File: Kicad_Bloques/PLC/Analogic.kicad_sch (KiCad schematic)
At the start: 1 part, among them U5 LM324A

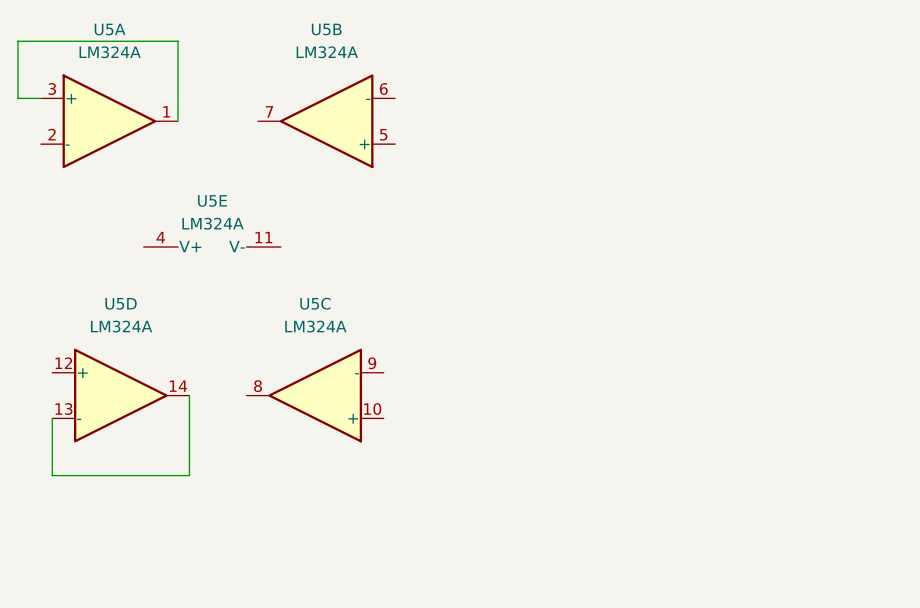
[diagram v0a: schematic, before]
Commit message: Bloque Analogico
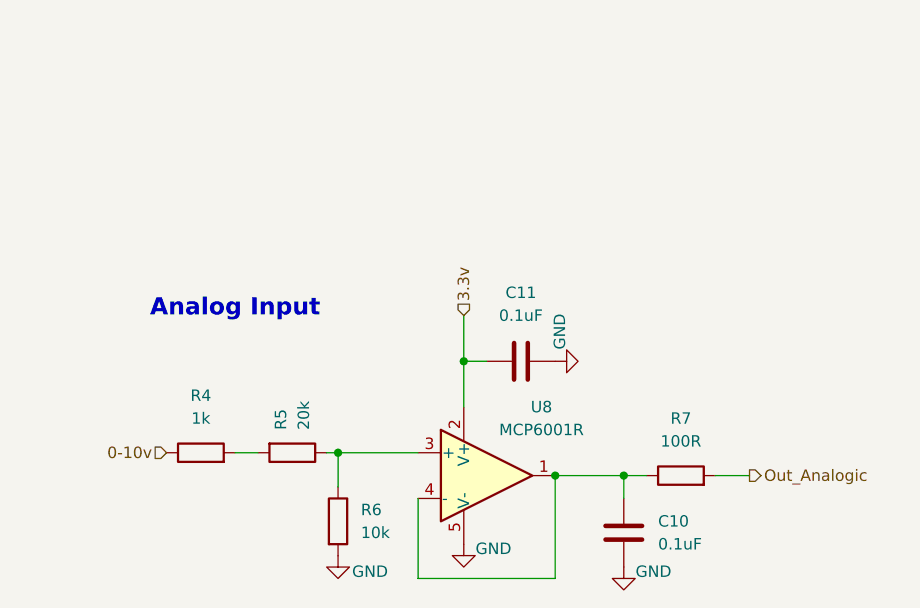
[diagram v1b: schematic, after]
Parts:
- removed U5: LM324A, symbol Amplifier_Operational:LM324A
- added C10, C11: 0.1uF, symbol Device:C
- added R4: 1k, symbol Device:R
- added R5: 20k, symbol Device:R
- added R6: 10k, symbol Device:R
- added R7: 100R, symbol Device:R
- added U8: MCP6001R, Package_TO_SOT_SMD:SOT-23-5, symbol Amplifier_Operational:MCP6001R
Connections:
- new net: C10.1, R7.1, U8.1, U8.4 (-)
- new net: R5.1, R6.1, U8.3 (+)
- new net: R4.2, R5.2
- new net 0-10v: R4.1
- new net 3.3v: C11.1, U8.2 (V+)
- new net GND: C10.2, C11.2, R6.2, U8.5 (V-)
- new net Out_Analogic: R7.2
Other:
- note added: "Analog Input"
